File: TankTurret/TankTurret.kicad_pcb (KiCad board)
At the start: 2 copper layers, 32 x 39.6 mm, 23 parts, among them J2 Camera, J3 SlipRing_6, P1 USB_C_Plug, U1 ESP32-WROVER-E

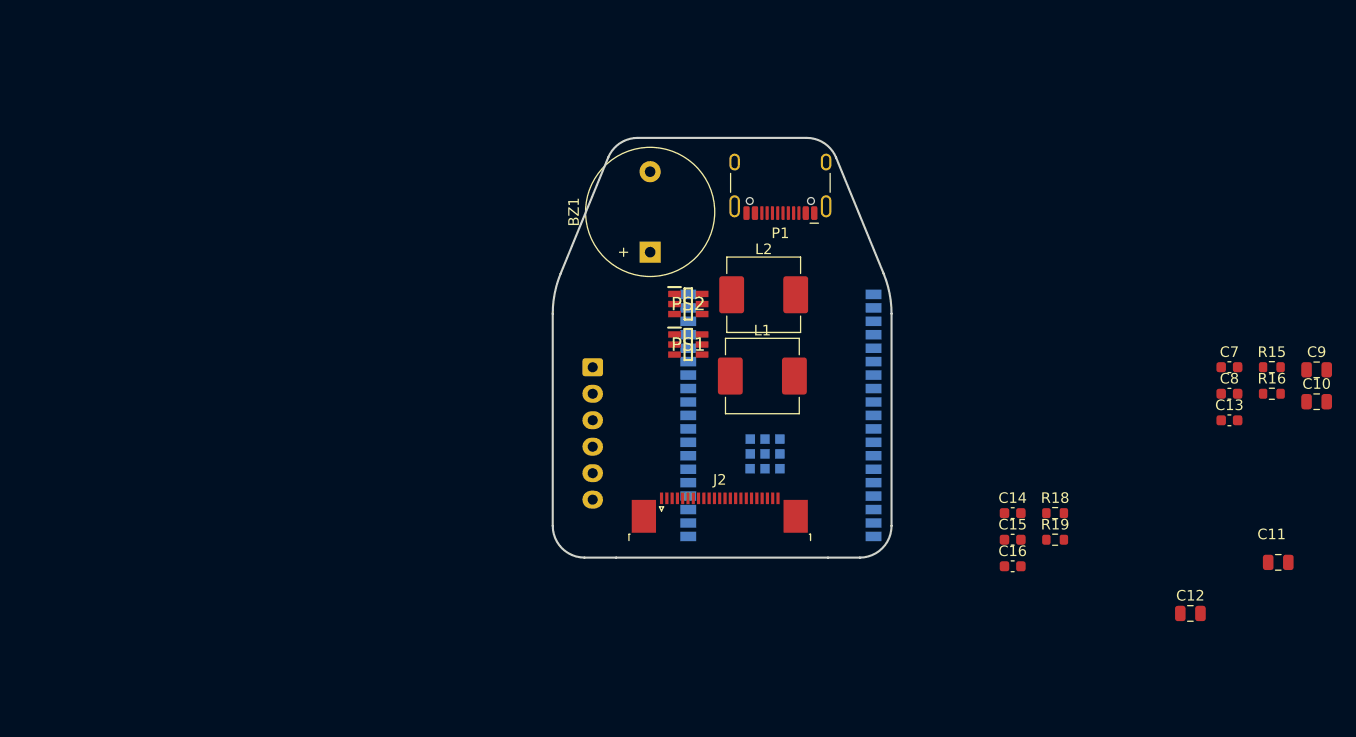
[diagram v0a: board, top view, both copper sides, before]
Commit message: camera connector
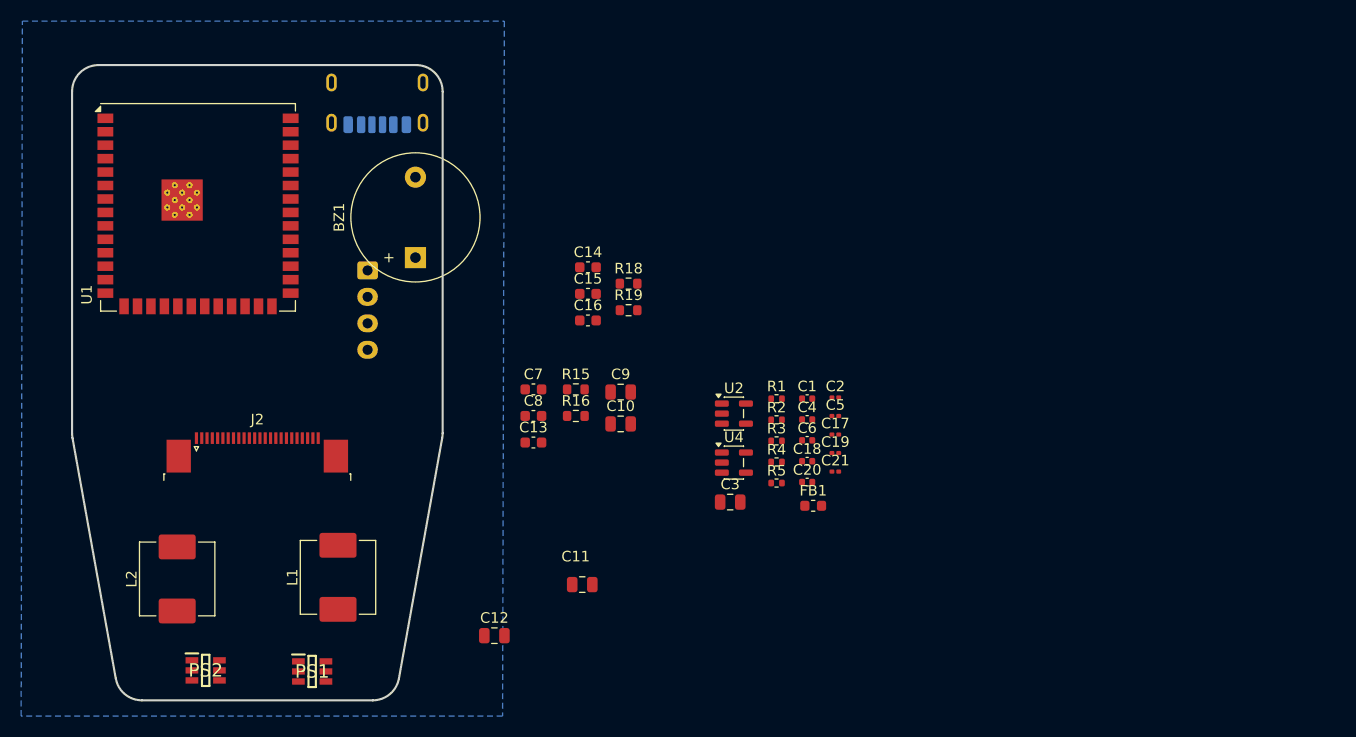
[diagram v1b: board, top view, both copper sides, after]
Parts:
- removed J3: SlipRing_6, Connector_JST:JST_XH_B6B-XH-A_1x06_P2.50mm_Vertical
- added C1: 100nF, Capacitor_SMD:C_0402_1005Metric, F.Cu at (123.3, 72.8)
- added C17: 1uF, Capacitor_SMD:C_0201_0603Metric, F.Cu at (125.9, 76.2)
- added C18: 100nF, Capacitor_SMD:C_0402_1005Metric, F.Cu at (123.3, 78.7)
- added C19: 1uF, Capacitor_SMD:C_0201_0603Metric, F.Cu at (125.9, 77.9)
- added C2: 1uF, Capacitor_SMD:C_0201_0603Metric, F.Cu at (125.9, 72.7)
- added C20: 100nF, Capacitor_SMD:C_0402_1005Metric, F.Cu at (123.3, 80.7)
- added C21: 1uF, Capacitor_SMD:C_0201_0603Metric, F.Cu at (125.9, 79.7)
- added C3: 4.7uF, Capacitor_SMD:C_0805_2012Metric, F.Cu at (116.0, 82.6)
- added C4: 100nF, Capacitor_SMD:C_0402_1005Metric, F.Cu at (123.3, 74.8)
- added C5: 1uF, Capacitor_SMD:C_0201_0603Metric, F.Cu at (125.9, 74.4)
- added C6: 100nF, Capacitor_SMD:C_0402_1005Metric, F.Cu at (123.3, 76.7)
- added FB1: FerriteBead, Inductor_SMD:L_0603_1608Metric, F.Cu at (123.8, 82.9)
- added J1: Conn_01x04_Socket, Connector_JST:JST_XH_B4B-XH-A_1x04_P2.50mm_Vertical, B.Cu at (81.7, 60.7)
- added R1: 4.7k, Resistor_SMD:R_0402_1005Metric, F.Cu at (120.4, 72.8)
- added R2: 4.7k, Resistor_SMD:R_0402_1005Metric, F.Cu at (120.4, 74.8)
- added R3: 10k, Resistor_SMD:R_0402_1005Metric, F.Cu at (120.4, 76.8)
- added R4: 10k, Resistor_SMD:R_0402_1005Metric, F.Cu at (120.4, 78.8)
- added R5: 33Ω, Resistor_SMD:R_0402_1005Metric, F.Cu at (120.4, 80.8)
- added U2: TLV70028_SOT353, Package_TO_SOT_SMD:SOT-23-5, F.Cu at (116.3, 74.2)
- added U4: TLV70012_SOT23-5, Package_TO_SOT_SMD:SOT-23-5, F.Cu at (116.3, 78.8)
- J2: footprint Connector_FFC-FPC:TE_2-1734839-3_1x23-1MP_P0.5mm_Horizontal -> Connector_FFC-FPC:TE_2-1734839-4_1x24-1MP_P0.5mm_Horizontal
- P1: footprint Connector_USB:USB_C_Receptacle_HCTL_HC-TYPE-C-16P-01A -> Connector_USB:USB_C_Receptacle_HRO_TYPE-C-31-M-17; moved to B.Cu
- U1: footprint PCM_Espressif:ESP32-WROVER-E -> RF_Module:ESP32-S3-WROOM-1U; moved to F.Cu
- moved C10 65.8 mm to (105.6, 75.2)
- moved C11 65.8 mm to (102.0, 90.3)
- moved C9 65.8 mm to (105.6, 72.2)
- moved R15 65.8 mm to (101.4, 71.9)
- moved R16 65.8 mm to (101.4, 74.4)
- moved C12 65.8 mm to (93.7, 95.2)
- moved C13 65.8 mm to (97.4, 76.9)
- moved C7 65.8 mm to (97.4, 71.9)
- moved C8 65.8 mm to (97.4, 74.4)
- moved L2 61.6 mm to (63.8, 89.8), turned to 90 degrees
- moved U1 59.6 mm to (65.7, 54.7)
- moved PS2 57.2 mm to (66.4, 98.5)
- moved PS1 47.1 mm to (76.5, 98.6)
- moved C14 46.3 mm to (102.6, 60.4)
- moved C15 46.3 mm to (102.6, 62.9)
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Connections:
- J2 pad 11: /GPIO34 -> /GPIO17
- J2 pad 12: /GPIO21 -> Net-(J2-XCLK)
- J2 pad 13: /GPIO35 -> /GPIO16
- J2 pad 14: unconnected-(J2-DOVDD-Pad14) -> +CAM_2V8
- J2 pad 15: unconnected-(J2-DVDD-Pad15) -> CAM_1V2
- J2 pad 16: /GPIO23 -> /GPIO7
- J2 pad 17: GND -> Net-(J2-PWDN)
- J2 pad 18: /GPIO25 -> /GPIO6
- J2 pad 20: /GPIO27 -> /GPIO5
- J2 pad 21: unconnected-(J2-AVDD-Pad21) -> Net-(J2-AVDD)
- J2 pad 22: /GPIO26 -> /GPIO4
- J2 pad 23: unconnected-(J2-AGND-Pad23) -> GND
- J2 pad 3: /GPIO18 -> /GPIO8
- J2 pad 4: /GPIO5 -> /GPIO9
- J2 pad 5: /GPIO19 -> /GPIO10
- J2 pad 6: /GPIO4 -> /GPIO11
- J2 pad 7: /GPIO36 -> /GPIO12
- J2 pad 8: /GPIO22 -> /GPIO13
- J2 pad 9: /GPIO39 -> /GPIO18
- U1 pad 1: GND -> Net-(U1-GND-Pad1)
- U1 pad 10: /GPIO25 -> unconnected-(U1-GPIO17/U1TXD/ADC2_CH6-Pad10)
- U1 pad 11: /GPIO26 -> unconnected-(U1-GPIO18/U1RXD/ADC2_CH7/CLK_OUT3-Pad11)
- U1 pad 12: /GPIO27 -> unconnected-(U1-GPIO8/TOUCH8/ADC1_CH7/SUBSPICS1-Pad12)
- U1 pad 13: /BUZZER -> unconnected-(U1-GPIO19/U1RTS/ADC2_CH8/CLK_OUT2/USB_D--Pad13)
- U1 pad 14: /IR #1 -> unconnected-(U1-GPIO20/U1CTS/ADC2_CH9/CLK_OUT1/USB_D+-Pad14)
- U1 pad 15: GND -> unconnected-(U1-GPIO3/TOUCH3/ADC1_CH2-Pad15)
- U1 pad 16: /TOP_LEDS -> unconnected-(U1-GPIO46-Pad16)
- U1 pad 17: (no net) -> unconnected-(U1-GPIO9/TOUCH9/ADC1_CH8/FSPIHD/SUBSPIHD-Pad17)
- U1 pad 18: (no net) -> unconnected-(U1-GPIO10/TOUCH10/ADC1_CH9/FSPICS0/FSPIIO4/SUBSPICS0-Pad18)
- U1 pad 19: (no net) -> unconnected-(U1-GPIO11/TOUCH11/ADC2_CH0/FSPID/FSPIIO5/SUBSPID-Pad19)
- U1 pad 20: (no net) -> unconnected-(U1-GPIO12/TOUCH12/ADC2_CH1/FSPICLK/FSPIIO6/SUBSPICLK-Pad20)
- U1 pad 21: (no net) -> unconnected-(U1-GPIO13/TOUCH13/ADC2_CH2/FSPIQ/FSPIIO7/SUBSPIQ-Pad21)
- U1 pad 22: (no net) -> unconnected-(U1-GPIO14/TOUCH14/ADC2_CH3/FSPIWP/FSPIDQS/SUBSPIWP-Pad22)
- U1 pad 24: /IR #2 -> unconnected-(U1-GPIO47/SPICLK_P/SUBSPICLK_P_DIFF-Pad24)
- U1 pad 26: /GPIO4 -> unconnected-(U1-GPIO45-Pad26)
- U1 pad 27: (no net) -> unconnected-(U1-GPIO0/BOOT-Pad27)
- U1 pad 28: (no net) -> unconnected-(U1-SPIIO6/GPIO35/FSPID/SUBSPID-Pad28)
- U1 pad 29: /GPIO5 -> unconnected-(U1-SPIIO7/GPIO36/FSPICLK/SUBSPICLK-Pad29)
- U1 pad 30: /GPIO18 -> unconnected-(U1-SPIDQS/GPIO37/FSPIQ/SUBSPIQ-Pad30)
- U1 pad 31: /GPIO19 -> unconnected-(U1-GPIO38/FSPIWP/SUBSPIWP-Pad31)
- U1 pad 32: (no net) -> unconnected-(U1-MTCK/GPIO39/CLK_OUT3/SUBSPICS1-Pad32)
- U1 pad 33: /GPIO21 -> unconnected-(U1-MTDO/GPIO40/CLK_OUT2-Pad33)
- U1 pad 34: /USB-UART RX -> unconnected-(U1-MTDI/GPIO41/CLK_OUT1-Pad34)
- U1 pad 35: /USB-UART TX -> unconnected-(U1-MTMS/GPIO42-Pad35)
- U1 pad 36: /GPIO22 -> unconnected-(U1-U0RXD/GPIO44/CLK_OUT2-Pad36)
- U1 pad 37: /GPIO23 -> unconnected-(U1-U0TXD/GPIO43/CLK_OUT1-Pad37)
- U1 pad 38: GND -> unconnected-(U1-GPIO2/TOUCH2/ADC1_CH1-Pad38)
- U1 pad 39: GND -> /BUZZER
- U1 pad 4: /GPIO36 -> unconnected-(U1-GPIO4/TOUCH4/ADC1_CH3-Pad4)
- U1 pad 5: /GPIO39 -> unconnected-(U1-GPIO5/TOUCH5/ADC1_CH4-Pad5)
- U1 pad 6: /GPIO34 -> unconnected-(U1-GPIO6/TOUCH6/ADC1_CH5-Pad6)
- U1 pad 7: /GPIO35 -> unconnected-(U1-GPIO7/TOUCH7/ADC1_CH6-Pad7)
- U1 pad 8: /I2C SCL -> unconnected-(U1-GPIO15/U0RTS/ADC2_CH4/XTAL_32K_P-Pad8)
- U1 pad 9: /I2C SDA -> unconnected-(U1-GPIO16/U0CTS/ADC2_CH5/XTAL_32K_N-Pad9)
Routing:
- added copper zone on B.Cu, net GND
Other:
- board size 32 x 39.6 mm -> 35 x 60 mm
